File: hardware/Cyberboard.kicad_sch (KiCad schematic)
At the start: 60 parts, among them CN1 B2B-XH-A (LF)(SN), J1 Conn_01x20, J2 Conn_01x20, SW1 SW_Push, SW2 SW_Push, U1 TPS630701RNMR, U2 NX2012SA-32.768KHZ-STD-MUB-2, U3 XL-1005UBC_C22355736, U5 BQ24074RGT, U6 STM32WB55CGUx, X1 NX2016SA-32MHZ-STD-CZS-5

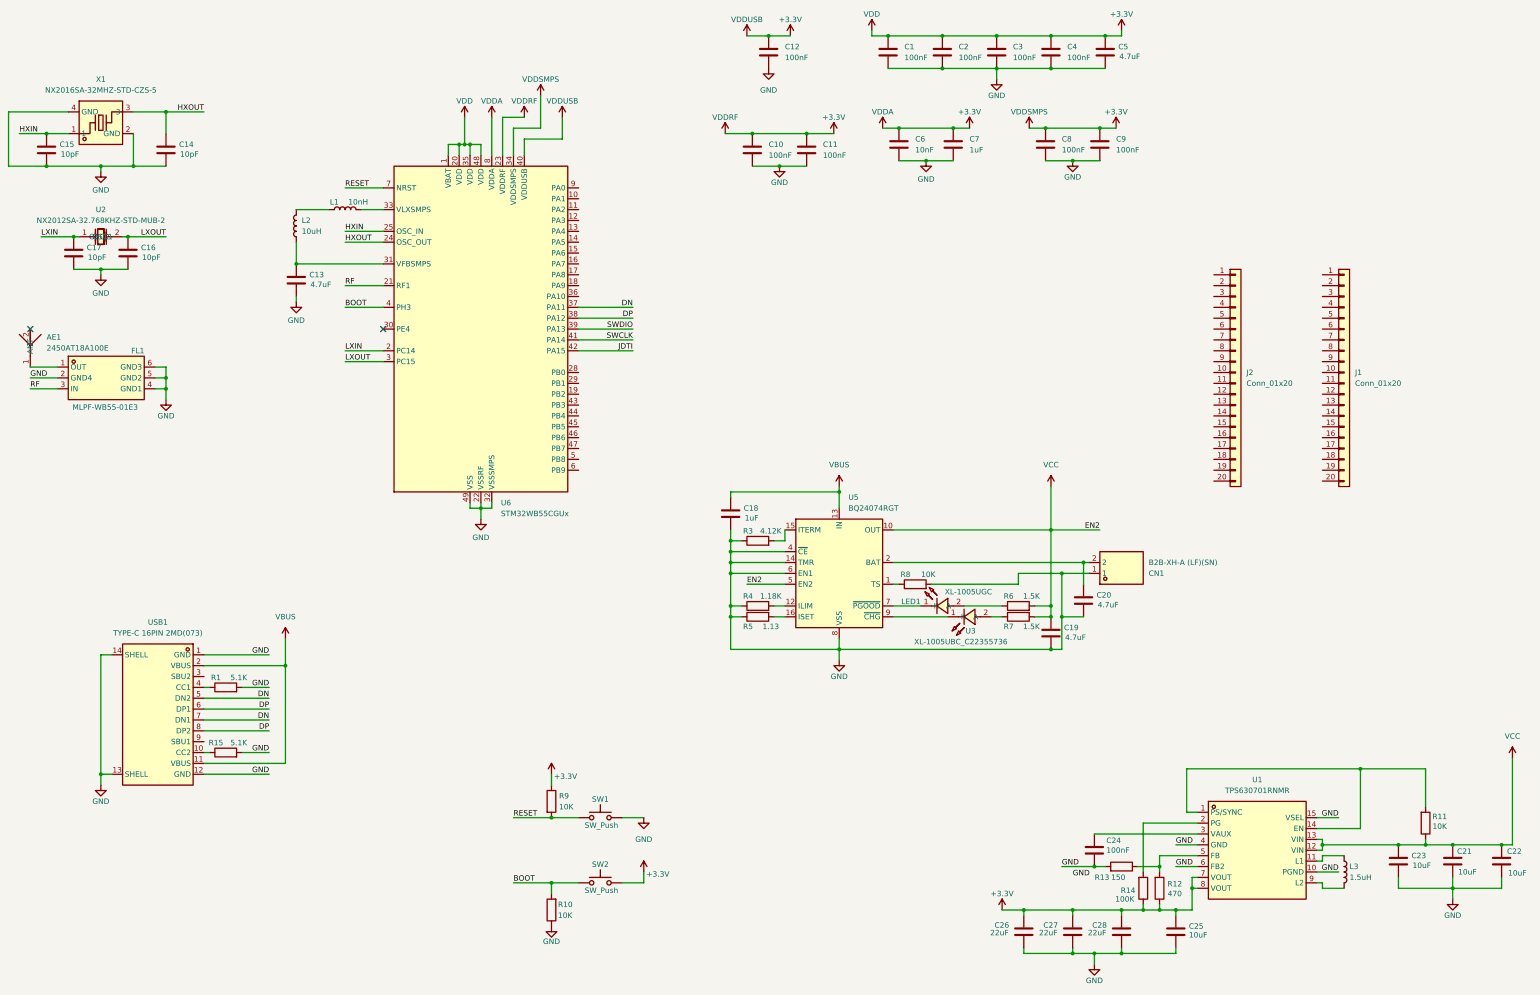
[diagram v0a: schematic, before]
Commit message: finished layout
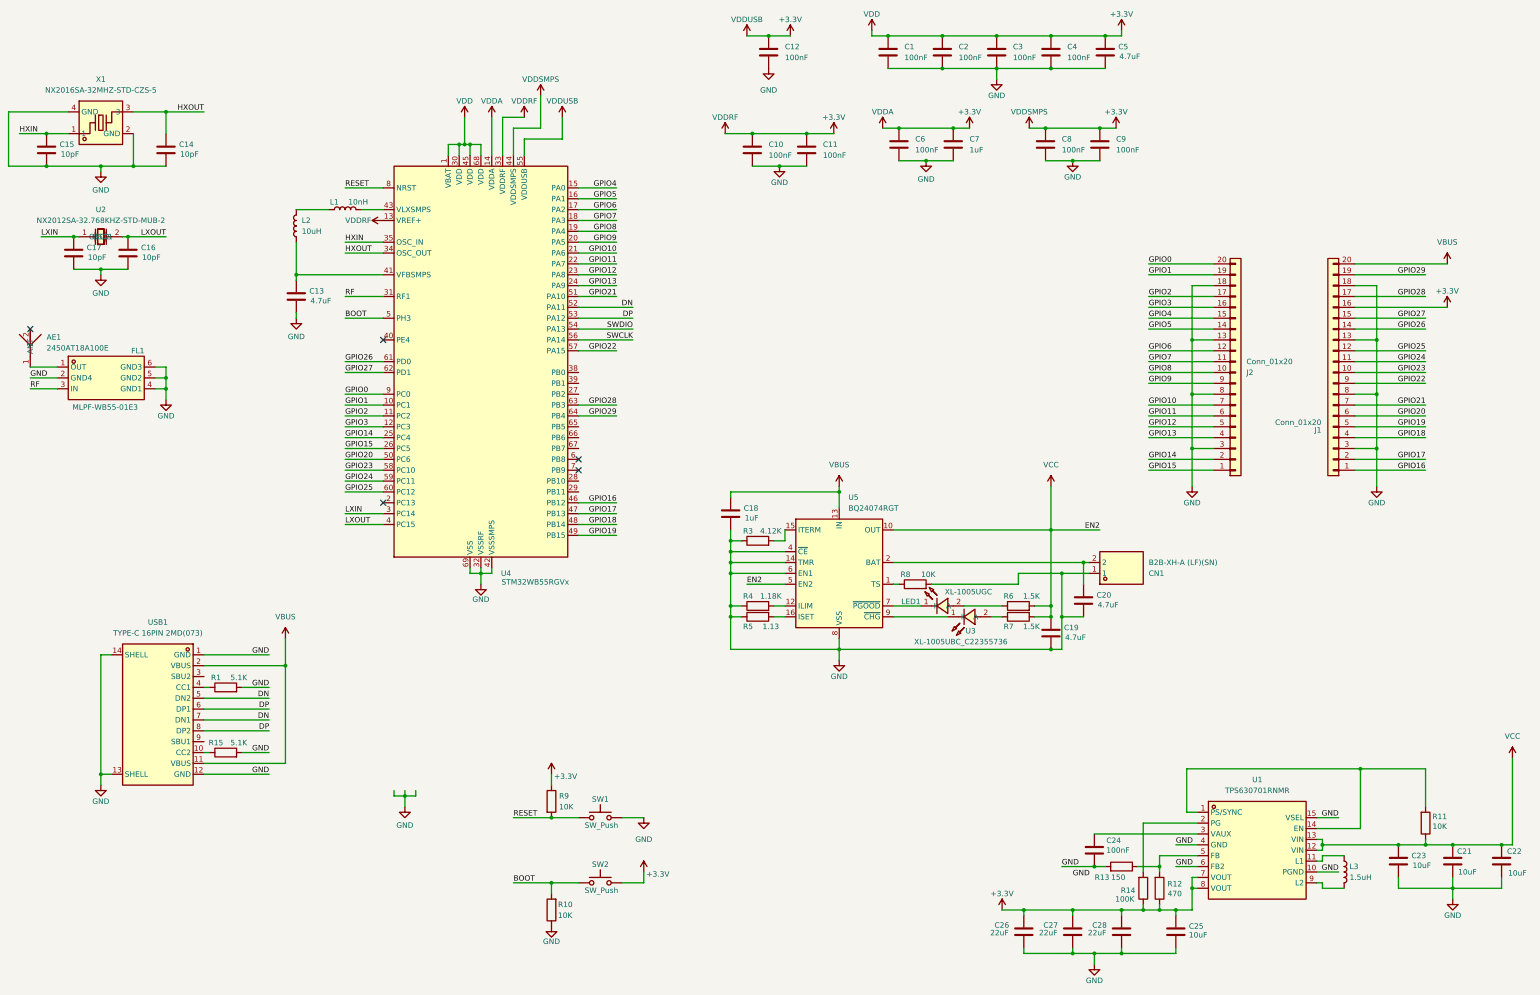
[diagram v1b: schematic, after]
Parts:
- removed U6: STM32WB55CGUx, Package_DFN_QFN:QFN-48-1EP_7x7mm_P0.5mm_EP5.6x5.6mm, symbol MCU_ST_STM32WB:STM32WB55CGUx
- added U4: STM32WB55RGVx, Package_DFN_QFN:QFN-68-1EP_8x8mm_P0.4mm_EP6.4x6.4mm, symbol MCU_ST_STM32WB:STM32WB55RGVx
- C21, C22, C25, C26, C27, C28: footprint Capacitor_SMD:C_0805_2012Metric -> Capacitor_SMD:C_0603_1608Metric
- C6: value 10nF -> 100nF
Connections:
- net +3.3V: now also J1.16 (Pin_16), U4.1 (VBAT), U4.13 (VREF+), U4.14 (VDDA), U4.30 (VDD), U4.33 (VDDRF), U4.44 (VDDSMPS), U4.45 (VDD), U4.55 (VDDUSB), U4.68 (VDD)
- net BOOT: now also U4.5 (PH3)
- net DN: now also U4.52 (PA11)
- net DP: now also U4.53 (PA12)
- net GND: now also J1.13 (Pin_13), J1.18 (Pin_18), J1.3 (Pin_3), J1.8 (Pin_8), J2.13 (Pin_13), J2.18 (Pin_18), J2.3 (Pin_3), J2.8 (Pin_8), U4.32 (VSSRF), U4.42 (VSSSMPS), U4.69 (VSS)
- net HXIN: now also U4.35 (OSC_IN)
- net HXOUT: now also U4.34 (OSC_OUT)
- net LXIN: now also U4.3 (PC14)
- net LXOUT: now also U4.4 (PC15)
- net RESET: now also U4.8 (NRST)
- net RF: now also U4.31 (RF1)
- net SWCLK: now also U4.56 (PA14)
- net SWDIO: now also U4.54 (PA13)
- net VBUS: now also J1.20 (Pin_20)
- net GPIO15: now reaches J2.1 (Pin_1)
- net GPIO15: now also U4.26 (PC5)
- net GPIO8: now reaches J2.10 (Pin_10)
- net GPIO8: now also U4.19 (PA4)
- net GPIO7: now reaches J2.11 (Pin_11)
- net GPIO7: now also U4.18 (PA3)
- net GPIO6: now reaches J2.12 (Pin_12)
- net GPIO6: now also U4.17 (PA2)
- net GPIO5: now reaches J2.14 (Pin_14)
- net GPIO5: now also U4.16 (PA1)
- net GPIO4: now reaches J2.15 (Pin_15)
- net GPIO4: now also U4.15 (PA0)
- net GPIO3: now reaches J2.16 (Pin_16)
- net GPIO3: now also U4.12 (PC3)
- net GPIO2: now reaches J2.17 (Pin_17)
- net GPIO2: now also U4.11 (PC2)
- net GPIO1: now reaches J2.19 (Pin_19)
- net GPIO1: now also U4.10 (PC1)
- net GPIO14: now reaches J2.2 (Pin_2)
- net GPIO14: now also U4.25 (PC4)
- net GPIO0: now reaches J2.20 (Pin_20)
- net GPIO0: now also U4.9 (PC0)
- net GPIO13: now reaches J2.4 (Pin_4)
- net GPIO13: now also U4.24 (PA9)
- net GPIO12: now reaches J2.5 (Pin_5)
- net GPIO12: now also U4.23 (PA8)
- net GPIO11: now reaches J2.6 (Pin_6)
- net GPIO11: now also U4.22 (PA7)
- net GPIO10: now reaches J2.7 (Pin_7)
- net GPIO10: now also U4.21 (PA6)
- net GPIO9: now reaches J2.9 (Pin_9)
- net GPIO9: now also U4.20 (PA5)
- net at L1.2: now also U4.43 (VLXSMPS)
- net GPIO16: now reaches J1.1 (Pin_1)
- net GPIO16: now also U4.46 (PB12)
- net GPIO23: now reaches J1.10 (Pin_10)
- net GPIO23: now also U4.58 (PC10)
- net GPIO24: now reaches J1.11 (Pin_11)
- net GPIO24: now also U4.59 (PC11)
- net GPIO25: now reaches J1.12 (Pin_12)
- net GPIO25: now also U4.60 (PC12)
- net GPIO26: now reaches J1.14 (Pin_14)
- net GPIO26: now also U4.61 (PD0)
- net GPIO27: now reaches J1.15 (Pin_15)
- net GPIO27: now also U4.62 (PD1)
- net GPIO28: now reaches J1.17 (Pin_17)
- net GPIO28: now also U4.63 (PB3)
- net GPIO29: now reaches J1.19 (Pin_19)
- net GPIO29: now also U4.64 (PB4)
- net GPIO17: now reaches J1.2 (Pin_2)
- net GPIO17: now also U4.47 (PB13)
- net GPIO18: now reaches J1.4 (Pin_4)
- net GPIO18: now also U4.48 (PB14)
- net GPIO19: now reaches J1.5 (Pin_5)
- net GPIO19: now also U4.49 (PB15)
- net GPIO20: now reaches J1.6 (Pin_6)
- net GPIO20: now also U4.50 (PC6)
- net GPIO21: now reaches J1.7 (Pin_7)
- net GPIO21: now also U4.51 (PA10)
- net GPIO22: now reaches J1.9 (Pin_9)
- net GPIO22: now also U4.57 (PA15)
- net at C13.1, L2.1: now also U4.41 (VFBSMPS)
- no-connect marks 2 -> 5
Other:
- moved on the sheet: C13, J1, J2
